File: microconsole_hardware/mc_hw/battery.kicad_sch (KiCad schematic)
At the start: 21 parts, among them J1 USB_C_Receptacle_USB2.0_16P, Q1 DMP2035U-7, Q2 DMP2035U-7, SW19 SPDT_Slide_PTH_11.6x4.0mm, U1 MCP73833-FCI/UN, U2 S2B-PH-K-S

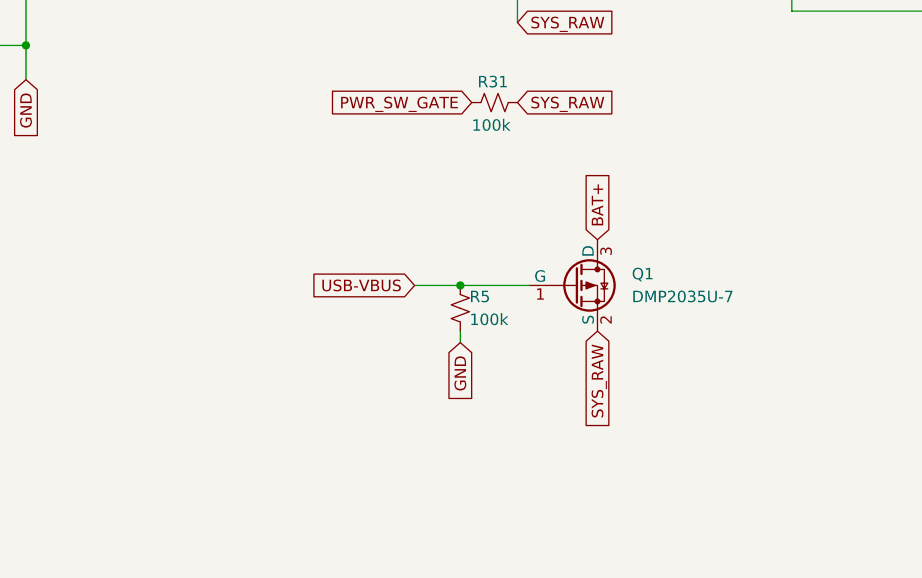
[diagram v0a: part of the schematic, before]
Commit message: fixup
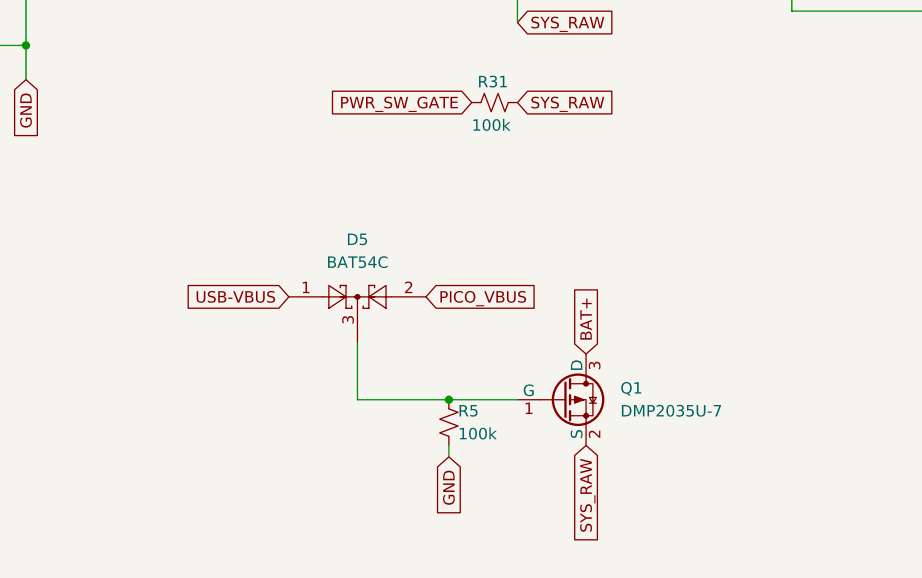
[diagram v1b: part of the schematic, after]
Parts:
- added D5: BAT54C, Package_TO_SOT_SMD:SOT-23, symbol Diode:BAT54C
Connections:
- net VDD: now also D5.1; no longer Q1.1 (G), R5.1
- new net: D5.3, Q1.1 (G), R5.1
- new net PICO_VBUS: D5.2
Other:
- moved on the sheet: Q1, R5

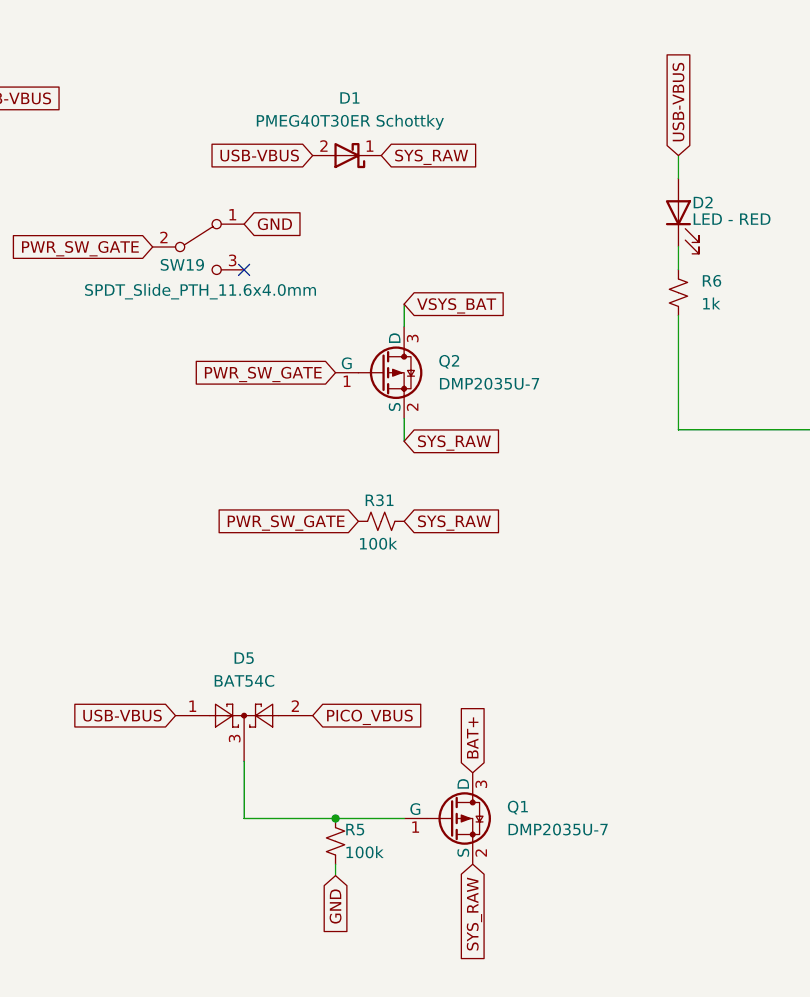
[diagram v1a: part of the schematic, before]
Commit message: fix up
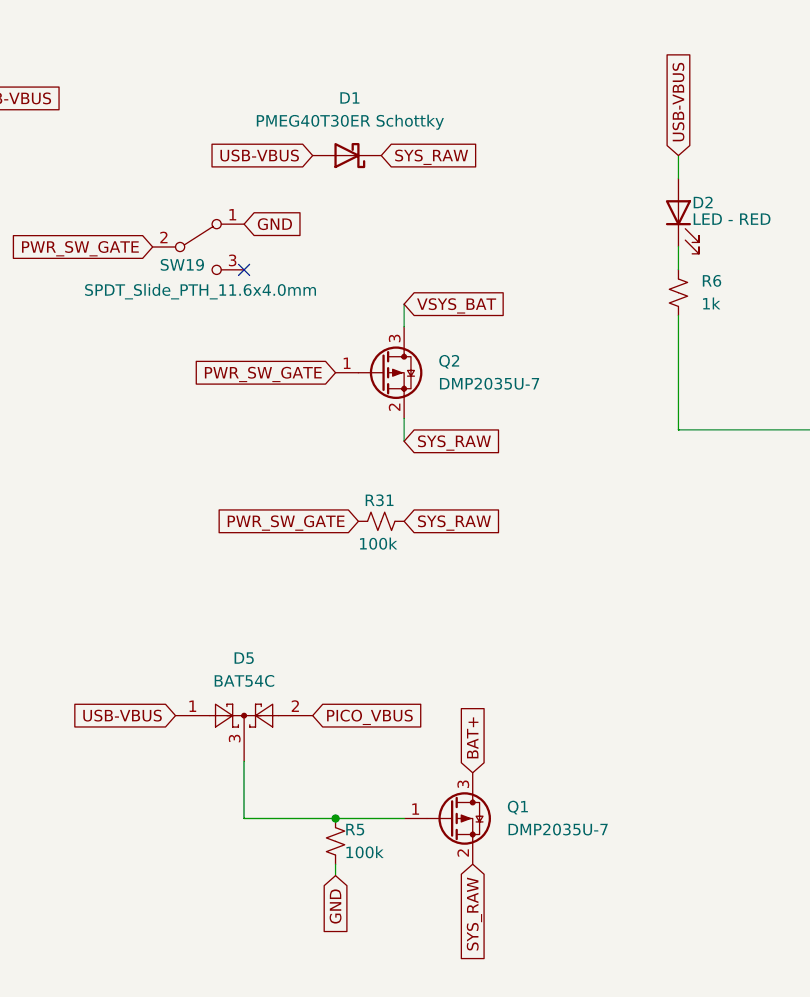
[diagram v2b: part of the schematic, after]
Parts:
- D1: footprint Diode_SMD:Nexperia_CFP3_SOD-123W -> (none)
- D2, D3, D4: footprint PCM_SparkFun-Resistor:R_0603_1608Metric -> (none)
- Q1, Q2: footprint Package_TO_SOT_SMD:SOT-23 -> (none)
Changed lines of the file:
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@@
 			)
 		)
-		(property "Footprint" "Diode_SMD:Nexperia_CFP3_SOD-123W"
+		(property "Footprint" ""
 			(at 120.65 38.1 0)
 			(hide yes)
@@
 			)
 		)
-		(property "Datasheet" "https://assets.nexperia.com/documents/data-sheet/PMEG40T30ER.pdf"
+		(property "Datasheet" ""
 			(at 120.65 38.1 0)
 			(hide yes)
@@
 			)
 		)
-		(property "Datasheet" "https://www.mouser.com/datasheet/3/282/1/22005b.pdf"
+		(property "Datasheet" "https://ww1.microchip.com/downloads/en/DeviceDoc/22005b.pdf"
 			(at 212.09 50.8 0)
 			(hide yes)
@@
 			)
 		)
-		(property "Footprint" "Package_TO_SOT_SMD:SOT-23"
+		(property "Footprint" ""
 			(at 137.16 109.22 0)
 			(hide yes)
@@
 			)
 		)
-		(property "Footprint" "PCM_SparkFun-Resistor:R_0603_1608Metric"
+		(property "Footprint" ""
 			(at 191.77 44.45 0)
 			(hide yes)
@@
 			)
 		)
-		(property "Footprint" "PCM_SparkFun-Resistor:R_0603_1608Metric"
+		(property "Footprint" ""
 			(at 157.48 44.45 0)
 			(hide yes)
@@
 			)
 		)
-		(property "Footprint" "PCM_SparkFun-Resistor:R_0603_1608Metric"
+		(property "Footprint" ""
 			(at 173.99 44.45 0)
 			(hide yes)
@@
 			)
 		)
-		(property "Footprint" "Package_TO_SOT_SMD:SOT-23"
+		(property "Footprint" ""
 			(at 129.54 59.69 0)
 			(hide yes)
